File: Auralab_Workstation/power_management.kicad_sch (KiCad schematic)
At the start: 20 parts, among them J1 USB_C_Receptacle_USB2.0_16P, U1 USBLC6-2SC6, U2 AP2112K-3.3, U3 TPS65131RGE

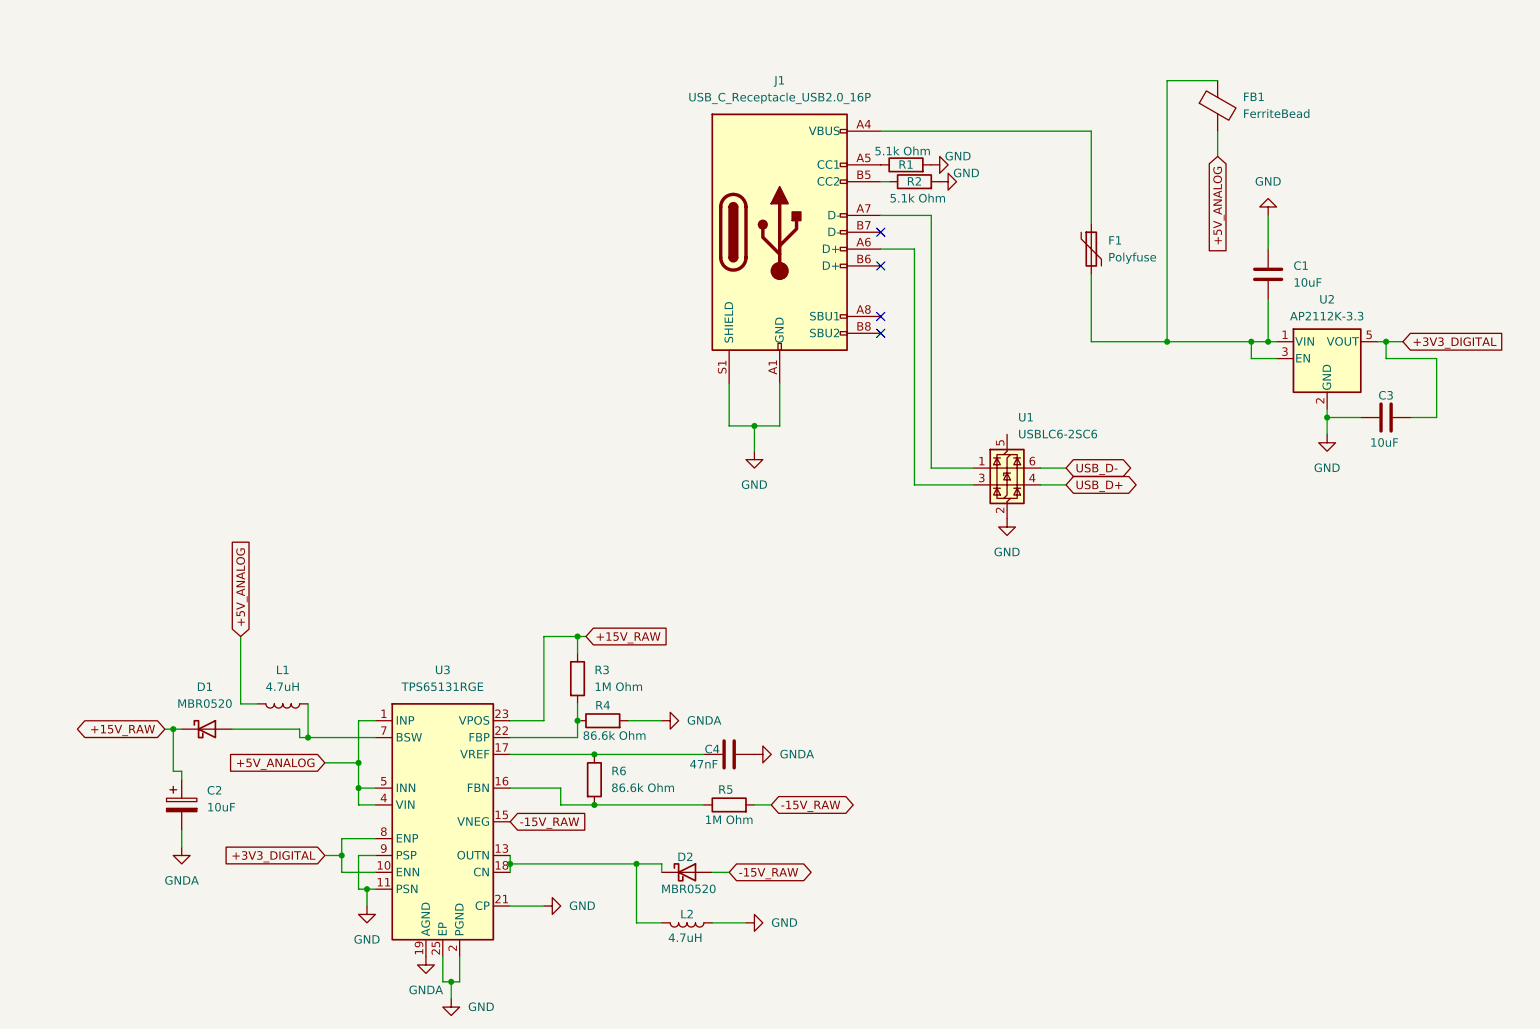
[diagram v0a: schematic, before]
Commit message: Power management le few changes made inum full ah complete panle..
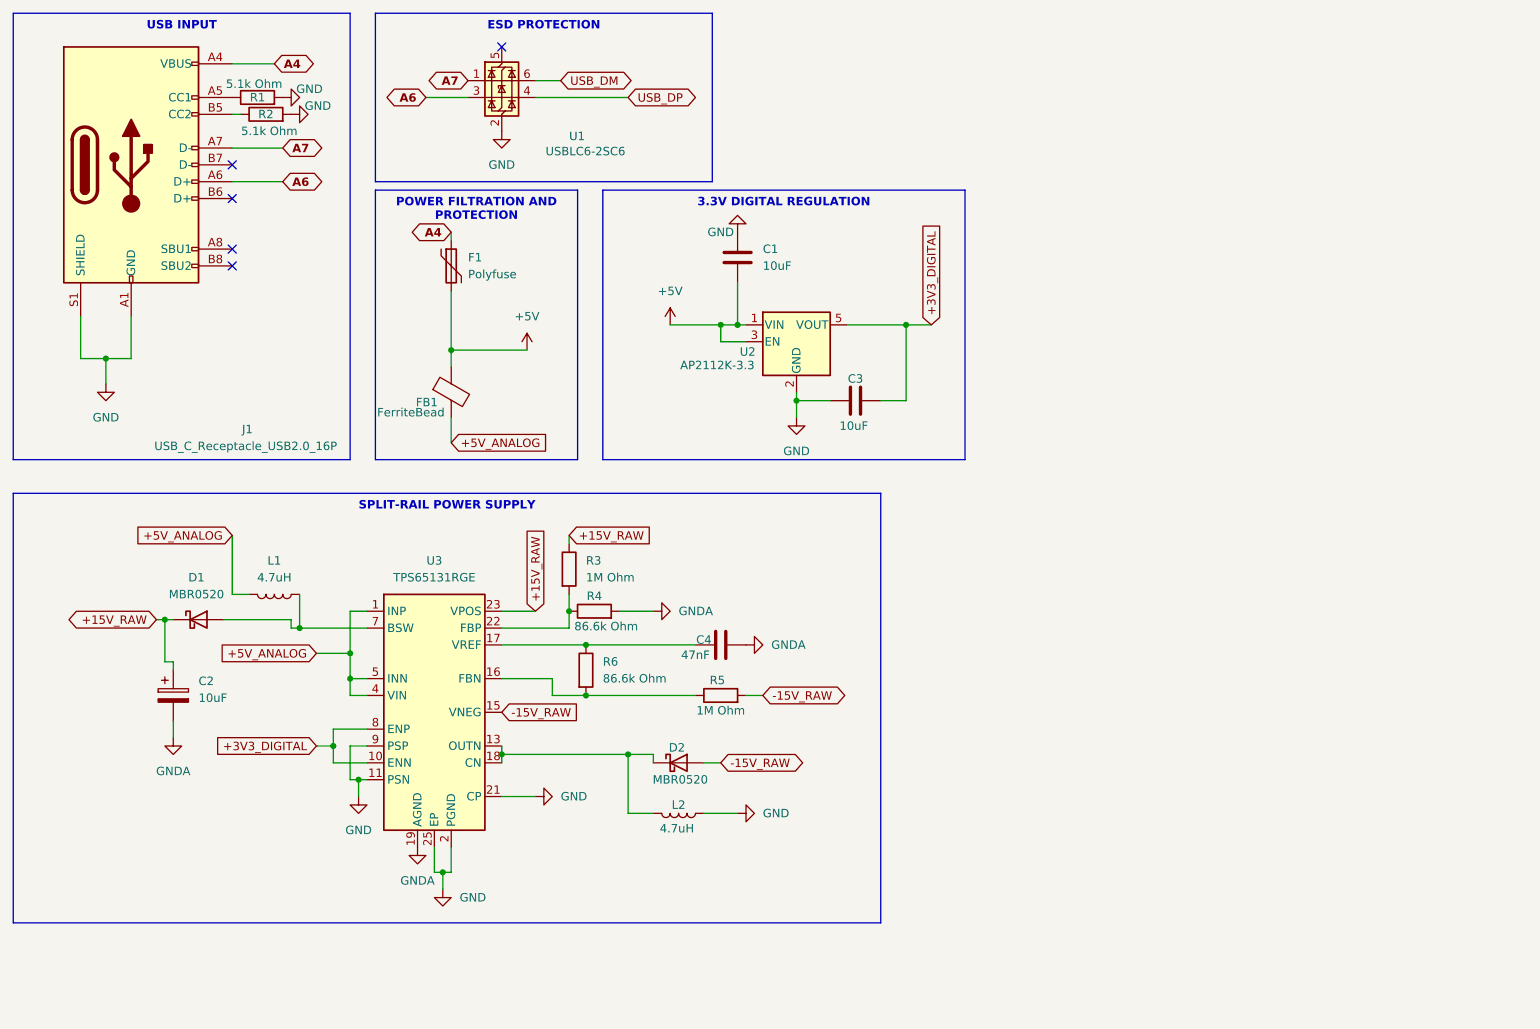
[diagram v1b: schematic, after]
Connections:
- net A4: now reaches F1.1, J1.A4 (VBUS), J1.A9 (VBUS), J1.B4 (VBUS), J1.B9 (VBUS)
- net +5V: now reaches C1.2, F1.2, FB1.1, U2.1 (VIN), U2.3 (EN)
- net A7: now reaches J1.A7 (D-), U1.1 (I/O1)
- net A6: now reaches J1.A6 (D+), U1.3 (I/O2)
- net USB_D+ renamed USB_DP
- net USB_D- renamed USB_DM
- no-connect marks 4 -> 5
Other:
- moved on the sheet: C1, C2, C3, C4, D1, D2, F1, FB1, J1, L1, L2, R1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
